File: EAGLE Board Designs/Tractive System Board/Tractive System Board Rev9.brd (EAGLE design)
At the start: 200 x 65 mm, 151 parts, among them K1 RELAY_SPST_NO_D_24, Q2 TRANSISTOR_N_MOS__PMV15ENEA, U1 OPAMP_1_CHANNEL_OPA991, U10 LTC6994-2, U5 RELAY_SOLIDSTATE_NO_AB38S-Q-A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, U6 LT8315, U7 AMC3330_AIRGAP, U8 AMC3330_AIRGAP

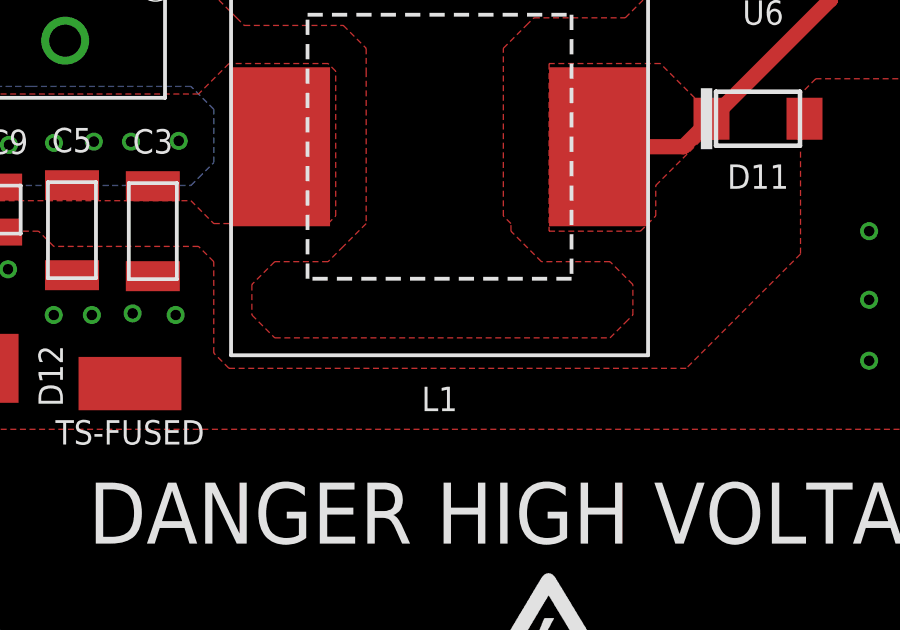
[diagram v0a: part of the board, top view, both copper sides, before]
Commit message: updated precharge relay
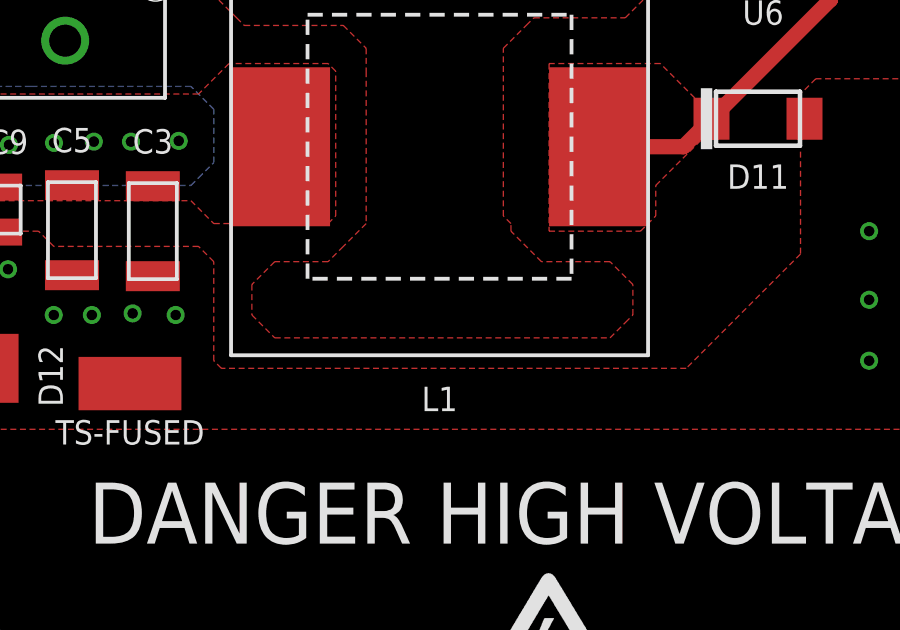
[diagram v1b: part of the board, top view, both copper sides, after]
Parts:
- K1: value RELAY_SPST_NO_D_24 -> RELAY_SPST_NO_D_200W_24
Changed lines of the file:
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@@
 <drawing>
 <settings>
-<setting alwaysvectorfont="no"/>
+<setting alwaysvectorfont="yes"/>
 <setting keepoldvectorfont="yes"/>
 <setting verticaltext="up"/>
@@
 <attribute name="NAME" x="44.704" y="-50.546" size="1.27" layer="25" font="vector" rot="R270" align="bottom-center"/>
 </element>
-<element name="K1" library="HyTechDevices" package="D" value="RELAY_SPST_NO_D_24" x="138.938" y="-46.99" smashed="yes" rot="R180">
-<attribute name="DKPN" value="725-1048-ND" x="95.758" y="-5.08" size="1.778" layer="27" rot="R180" display="off"/>
+<element name="K1" library="HyTechDevices" package="D" value="RELAY_SPST_NO_D_200W_24" x="138.938" y="-46.99" smashed="yes" rot="R180">
+<attribute name="DKPN" value="725-1362-ND" x="95.758" y="-5.08" size="1.778" layer="27" rot="R180" display="off"/>
 <attribute name="MANUFACTURER" value="Sensata-Cynergy3" x="95.758" y="-5.08" size="1.778" layer="27" rot="R180" display="off"/>
-<attribute name="MOPN" value="285-DAR72410" x="95.758" y="-5.08" size="1.778" layer="27" rot="R180" display="off"/>
-<attribute name="MPN" value="DAR72410" x="95.758" y="-5.08" size="1.778" layer="27" rot="R180" display="off"/>
+<attribute name="MOPN" value="285-DAT200-24" x="95.758" y="-5.08" size="1.778" layer="27" rot="R180" display="off"/>
+<attribute name="MPN" value="DAT200-24" x="95.758" y="-5.08" size="1.778" layer="27" rot="R180" display="off"/>
 <attribute name="NAME" x="169.9" y="-47.018" size="0.8128" layer="21" font="vector" rot="R270" align="bottom-center"/>
 </element>
@@
 <vertex x="55.88" y="-21.59"/>
 <vertex x="52.07" y="-25.4"/>
-<vertex x="36.83" y="-25.4"/>
-<vertex x="36.322" y="-24.892"/>
+<vertex x="36.576" y="-25.4"/>
+<vertex x="36.322" y="-25.146"/>
 <vertex x="36.322" y="-21.844"/>
 <vertex x="35.814" y="-21.336"/>
